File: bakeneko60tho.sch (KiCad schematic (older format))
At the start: 160 parts, among them J1 Conn_01x04_Male, SW1 SW_Push, Y1 16MHz

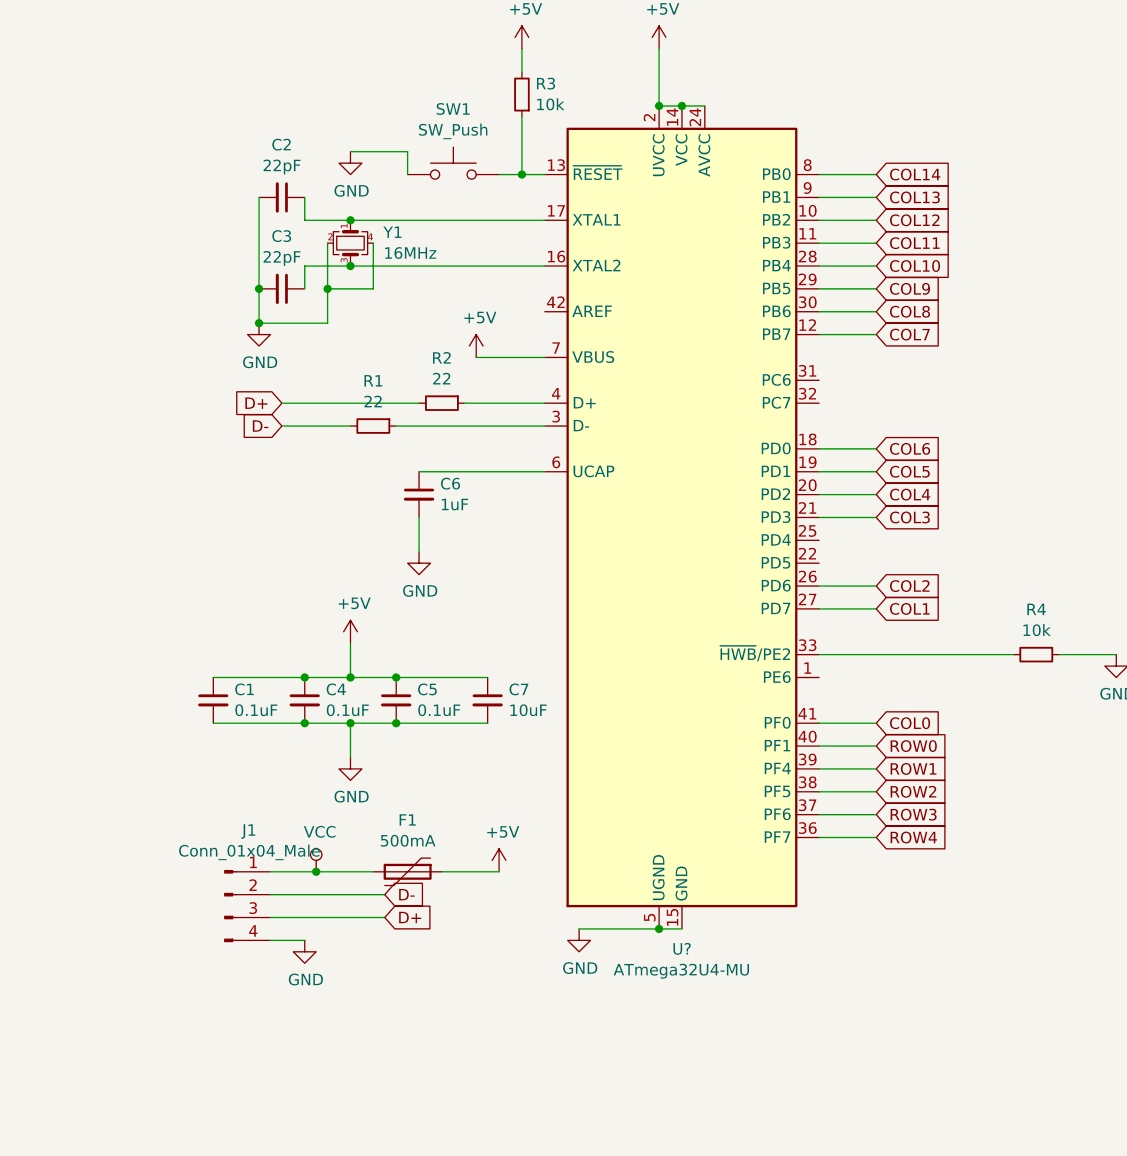
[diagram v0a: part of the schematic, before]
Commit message: complete routing
finishing the routing
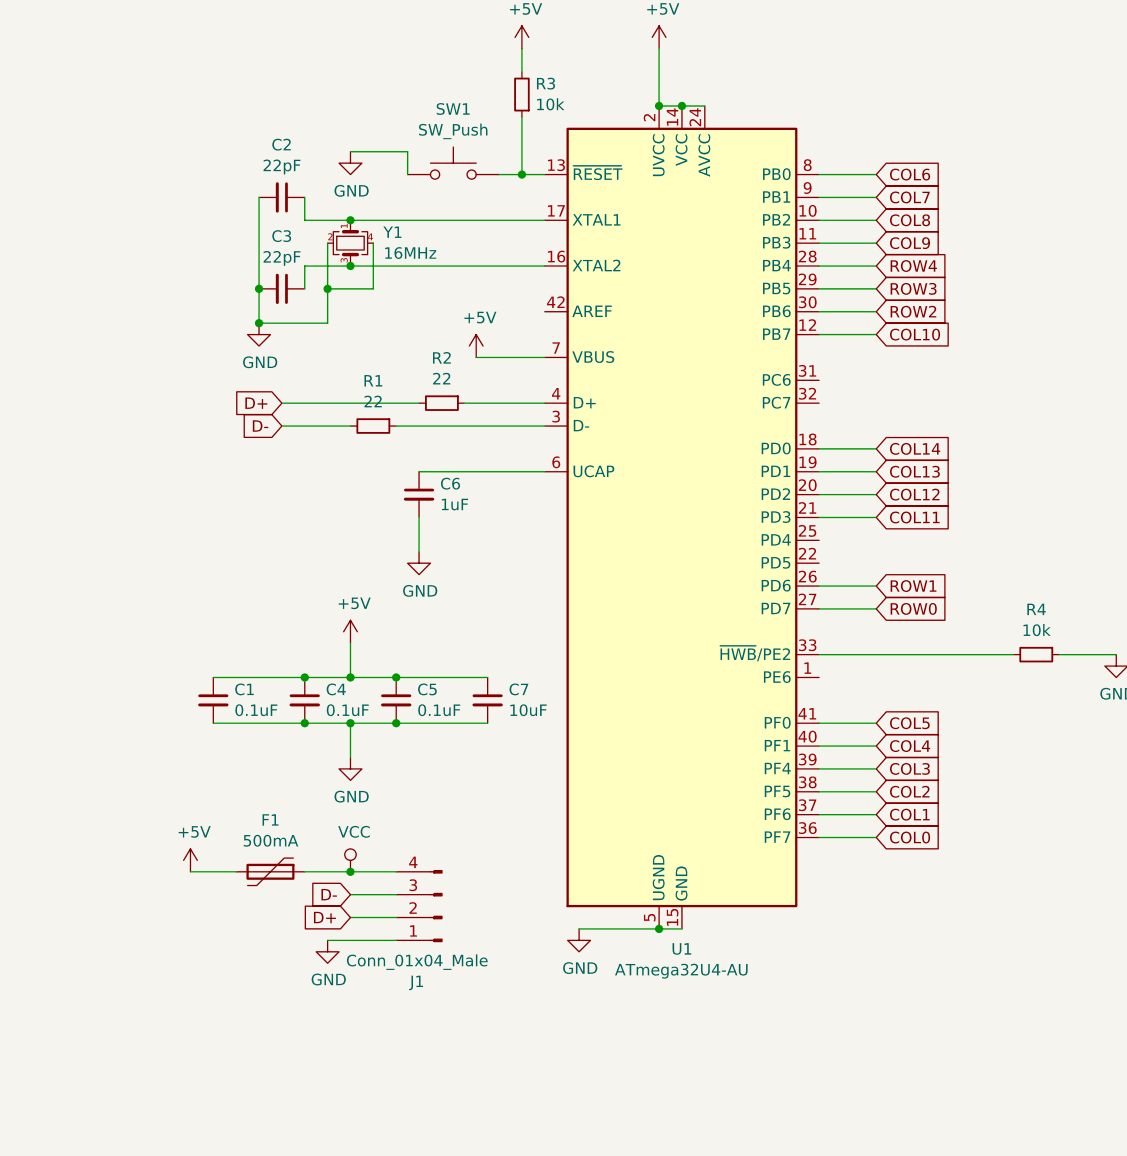
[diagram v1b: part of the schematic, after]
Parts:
- removed U?: ATmega32U4-MU, Package_DFN_QFN:QFN-44-1EP_7x7mm_P0.5mm_EP5.2x5.2mm, symbol MCU_Microchip_ATmega:ATmega32U4-MU
- added U1: ATmega32U4-AU, Package_QFP:TQFP-44_10x10mm_P0.8mm, symbol MCU_Microchip_ATmega:ATmega32U4-AU
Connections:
- net +5V: now also F1.2, U1.14 (VCC), U1.2 (UVCC), U1.24 (AVCC), U1.34 (VCC), U1.44 (AVCC), U1.7 (VBUS); no longer F1.1
- net COL0: now also U1.36 (PF7)
- net COL1: now also U1.37 (PF6)
- net COL10: now also U1.12 (PB7)
- net COL11: now also U1.21 (PD3)
- net COL12: now also U1.20 (PD2)
- net COL13: now also U1.19 (PD1)
- net COL14: now also U1.18 (PD0)
- net COL2: now also U1.38 (PF5)
- net COL3: now also U1.39 (PF4)
- net COL4: now also U1.40 (PF1)
- net COL5: now also U1.41 (PF0)
- net COL6: now also U1.8 (PB0)
- net COL7: now also U1.9 (PB1)
- net COL8: now also U1.10 (PB2)
- net COL9: now also U1.11 (PB3)
- net D+: now also J1.2 (Pin_2); no longer J1.3 (Pin_3)
- net D-: now also J1.3 (Pin_3); no longer J1.2 (Pin_2)
- net GND: now also J1.1 (Pin_1), U1.15 (GND), U1.23 (GND), U1.35 (GND), U1.43 (GND), U1.5 (UGND); no longer J1.4 (Pin_4)
- net ROW0: now also U1.27 (PD7)
- net ROW1: now also U1.26 (PD6)
- net ROW2: now also U1.30 (PB6)
- net ROW3: now also U1.29 (PB5)
- net ROW4: now also U1.28 (PB4)
- net VCC: now also F1.1, J1.4 (Pin_4); no longer F1.2, J1.1 (Pin_1)
- net at R4.2: now also U1.33 (~HWB~/PE2)
- net at R2.1: now also U1.4 (D+)
- net at R1.1: now also U1.3 (D-)
- net at C6.1: now also U1.6 (UCAP)
- net at C2.1, Y1.1: now also U1.17 (XTAL1)
- net at C3.1, Y1.3: now also U1.16 (XTAL2)
- net at R3.1, SW1.2: now also U1.13 (~RESET)
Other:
- moved on the sheet: F1, J1

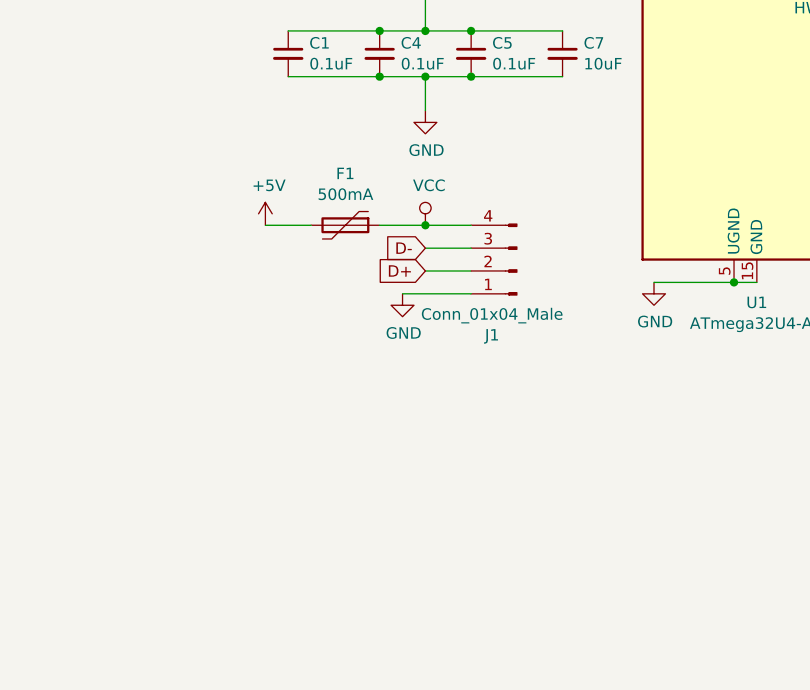
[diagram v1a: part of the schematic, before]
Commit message: fix routing
fix routing bugs
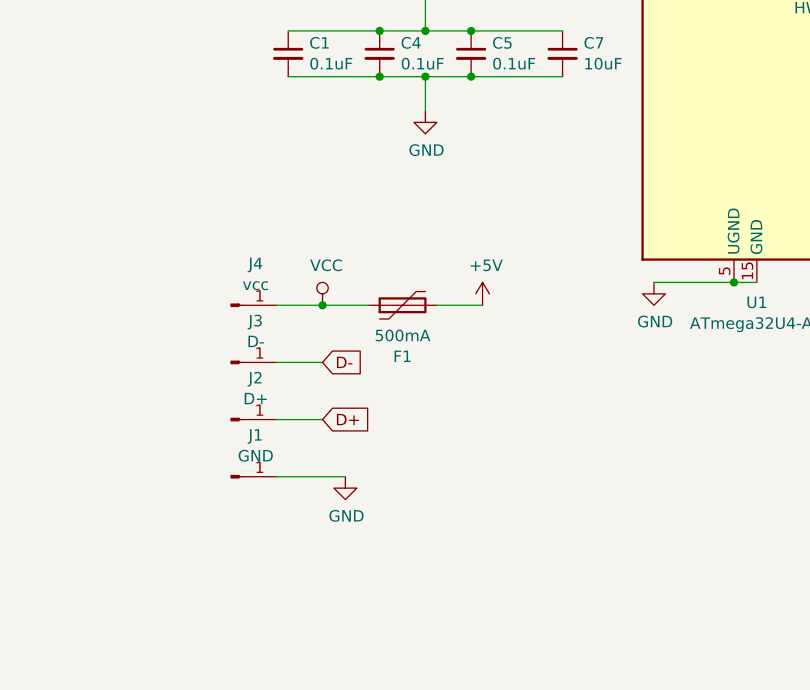
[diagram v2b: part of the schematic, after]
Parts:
- removed J1: Conn_01x04_Male, Connector_PinHeader_1.00mm:PinHeader_1x04_P1.00mm_Horizontal, symbol Connector:Conn_01x04_Male
- added J1: GND, Connector_PinHeader_1.00mm:PinHeader_1x01_P1.00mm_Vertical, symbol Connector:Conn_01x01_Male
- added J2: D+, Connector_PinHeader_1.00mm:PinHeader_1x01_P1.00mm_Vertical, symbol Connector:Conn_01x01_Male
- added J3: D-, Connector_PinHeader_1.00mm:PinHeader_1x01_P1.00mm_Vertical, symbol Connector:Conn_01x01_Male
- added J4: vcc, Connector_PinHeader_1.00mm:PinHeader_1x01_P1.00mm_Vertical, symbol Connector:Conn_01x01_Male
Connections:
- net D+: now also J2.1 (Pin_1)
- net D-: now also J3.1 (Pin_1)
- net GND: now also J1.1 (Pin_1)
- net VCC: now also J4.1 (Pin_1)
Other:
- moved on the sheet: F1
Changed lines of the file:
@@
 L power:+5V #PWR0111
 U 1 1 62850546
-P 6550 4750
-F 0 "#PWR0111" H 6550 4600 50  0001 C CNN
-F 1 "+5V" H 6565 4923 50  0000 C CNN
-F 2 "" H 6550 4750 50  0001 C CNN
-F 3 "" H 6550 4750 50  0001 C CNN
-	1    6550 4750
+P 7500 5100
+F 0 "#PWR0111" H 7500 4950 50  0001 C CNN
+F 1 "+5V" H 7515 5273 50  0000 C CNN
+F 2 "" H 7500 5100 50  0001 C CNN
+F 3 "" H 7500 5100 50  0001 C CNN
+	1    7500 5100
 	1    0    0    -1
 $EndComp
@@
 L Device:Polyfuse F1
 U 1 1 6284E1C3
-P 6900 4750
-F 0 "F1" V 6675 4750 50  0000 C CNN
-F 1 "500mA" V 6766 4750 50  0000 C CNN
-F 2 "Fuse:Fuse_1206_3216Metric" H 6950 4550 50  0001 L CNN
-F 3 "~" H 6900 4750 50  0001 C CNN
-	1    6900 4750
-	0    1    1    0
+P 7150 5100
+F 0 "F1" V 6925 5100 50  0000 C CNN
+F 1 "500mA" V 7016 5100 50  0000 C CNN
+F 2 "Fuse:Fuse_1206_3216Metric" H 7200 4900 50  0001 L CNN
+F 3 "~" H 7150 5100 50  0001 C CNN
+	1    7150 5100
+	0    -1   -1   0
 $EndComp
 $Comp
 L power:VCC #PWR0112
 U 1 1 6284D4F2
-P 7250 4750
-F 0 "#PWR0112" H 7250 4600 50  0001 C CNN
-F 1 "VCC" H 7267 4923 50  0000 C CNN
-F 2 "" H 7250 4750 50  0001 C CNN
-F 3 "" H 7250 4750 50  0001 C CNN
-	1    7250 4750
-	1    0    0    -1
-$EndComp
-$Comp
-L Connector:Conn_01x04_Male J1
-U 1 1 6288D02A
-P 7650 4950
-F 0 "J1" H 7758 5231 50  0000 C CNN
-F 1 "Conn_01x04_Male" H 7758 5140 50  0000 C CNN
-F 2 "Connector_PinHeader_1.00mm:PinHeader_1x04_P1.00mm_Horizontal" H 7650 4950 50  0001 C CNN
-F 3 "~" H 7650 4950 50  0001 C CNN
-	1    7650 4950
-	-1   0    0    1
-$EndComp
-Text GLabel 7250 4950 0    50   Input ~ 0
-D+
-Text GLabel 7250 4850 0    50   Input ~ 0
-D-
+P 6800 5100
+F 0 "#PWR0112" H 6800 4950 50  0001 C CNN
+F 1 "VCC" H 6817 5273 50  0000 C CNN
+F 2 "" H 6800 5100 50  0001 C CNN
+F 3 "" H 6800 5100 50  0001 C CNN
+	1    6800 5100
+	1    0    0    -1
+$EndComp
 $Comp
 L power:GND #PWR0113
 U 1 1 628948D3
-P 7150 5050
-F 0 "#PWR0113" H 7150 4800 50  0001 C CNN
-F 1 "GND" H 7155 4877 50  0000 C CNN
-F 2 "" H 7150 5050 50  0001 C CNN
-F 3 "" H 7150 5050 50  0001 C CNN
-	1    7150 5050
+P 6900 5850
+F 0 "#PWR0113" H 6900 5600 50  0001 C CNN
+F 1 "GND" H 6905 5677 50  0000 C CNN
+F 2 "" H 6900 5850 50  0001 C CNN
+F 3 "" H 6900 5850 50  0001 C CNN
+	1    6900 5850
 	1    0    0    -1
 $EndComp
@@
 ROW0
 Wire Wire Line
-	7150 5050 7450 5050
-Wire Wire Line
-	7250 4950 7450 4950
-Wire Wire Line
-	7250 4850 7450 4850
-Wire Wire Line
-	6550 4750 6750 4750
-Wire Wire Line
-	7050 4750 7250 4750
-Wire Wire Line
-	7250 4750 7450 4750
-Connection ~ 7250 4750
+	6900 5850 6600 5850
+Wire Wire Line
+	7500 5100 7300 5100
+Wire Wire Line
+	7000 5100 6800 5100
+Wire Wire Line
+	6800 5100 6600 5100
+Connection ~ 6800 5100
 Wire Wire Line
 	8600 1400 8700 1400
@@
 Wire Wire Line
 	9300 4600 9550 4600
+$Comp
+L Connector:Conn_01x01_Male J4
+U 1 1 62DF2DF2
+P 6400 5100
+F 0 "J4" H 6508 5281 50  0000 C CNN
+F 1 "vcc" H 6508 5190 50  0000 C CNN
+F 2 "Connector_PinHeader_1.00mm:PinHeader_1x01_P1.00mm_Vertical" H 6400 5100 50  0001 C CNN
+F 3 "~" H 6400 5100 50  0001 C CNN
+	1    6400 5100
+	1    0    0    -1
+$EndComp
+$Comp
+L Connector:Conn_01x01_Male J1
+U 1 1 62DF4B11
+P 6400 5850
+F 0 "J1" H 6508 6031 50  0000 C CNN
+F 1 "GND" H 6508 5940 50  0000 C CNN
+F 2 "Connector_PinHeader_1.00mm:PinHeader_1x01_P1.00mm_Vertical" H 6400 5850 50  0001 C CNN
+F 3 "~" H 6400 5850 50  0001 C CNN
+	1    6400 5850
+	1    0    0    -1
+$EndComp
+$Comp
+L Connector:Conn_01x01_Male J3
+U 1 1 62DF471A
+P 6400 5350
+F 0 "J3" H 6508 5531 50  0000 C CNN
+F 1 "D-" H 6508 5440 50  0000 C CNN
+F 2 "Connector_PinHeader_1.00mm:PinHeader_1x01_P1.00mm_Vertical" H 6400 5350 50  0001 C CNN
+F 3 "~" H 6400 5350 50  0001 C CNN
+	1    6400 5350
+	1    0    0    -1
+$EndComp
+Wire Wire Line
+	6600 5350 6800 5350
+Text GLabel 6800 5350 2    50   Input ~ 0
+D-
+$Comp
+L Connector:Conn_01x01_Male J2
+U 1 1 62DF4913
+P 6400 5600
+F 0 "J2" H 6508 5781 50  0000 C CNN
+F 1 "D+" H 6508 5690 50  0000 C CNN
+F 2 "Connector_PinHeader_1.00mm:PinHeader_1x01_P1.00mm_Vertical" H 6400 5600 50  0001 C CNN
+F 3 "~" H 6400 5600 50  0001 C CNN
+	1    6400 5600
+	1    0    0    -1
+$EndComp
+Wire Wire Line
+	6800 5600 6600 5600
+Text GLabel 6800 5600 2    50   Input ~ 0
+D+
 $EndSCHEMATC
